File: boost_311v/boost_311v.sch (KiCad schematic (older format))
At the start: 58 parts, among them J2 VO, J3 Vin_boost, Q1 BC556, Q2 PN2222A, Q3 PN2222A, Q4 PN2222A, Q5 IRFP260, Q6 2N3904, Q7 2N3906, U2 L7812, U3 4N25, U4 LF357, U5 NE555

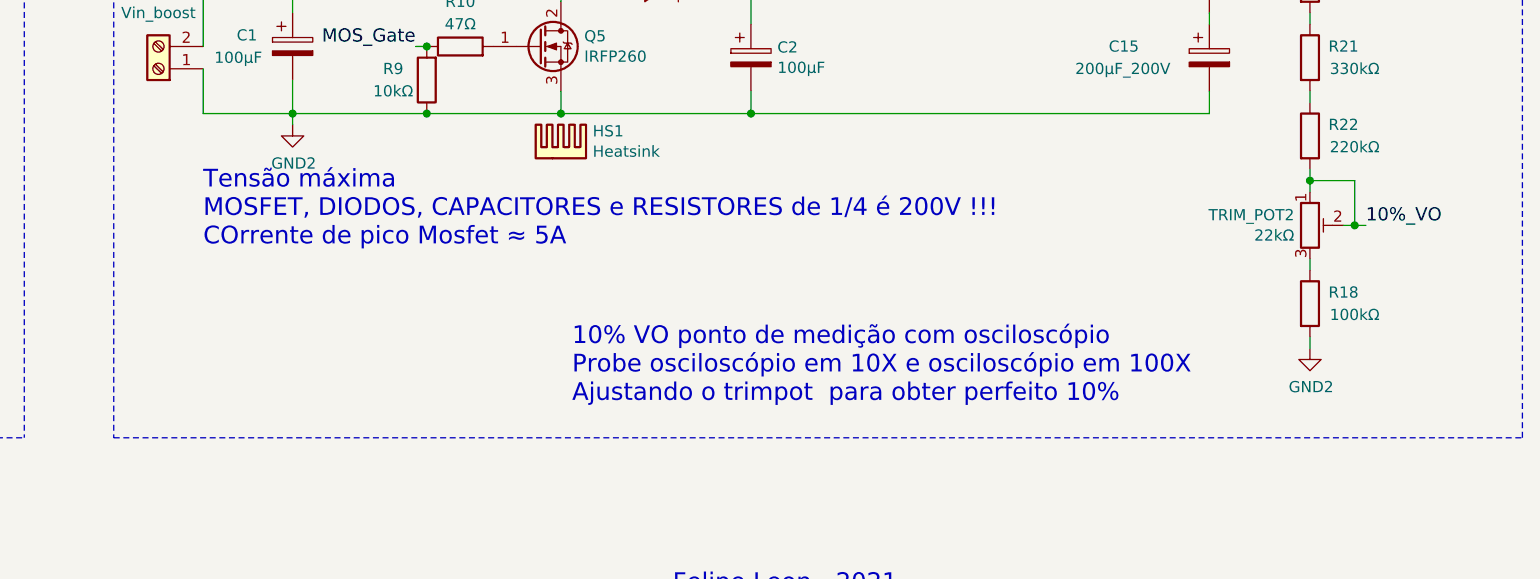
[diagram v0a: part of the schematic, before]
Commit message: Up pcb
Signed-off-by: fgl27 <fglfgl27@gmail.com>
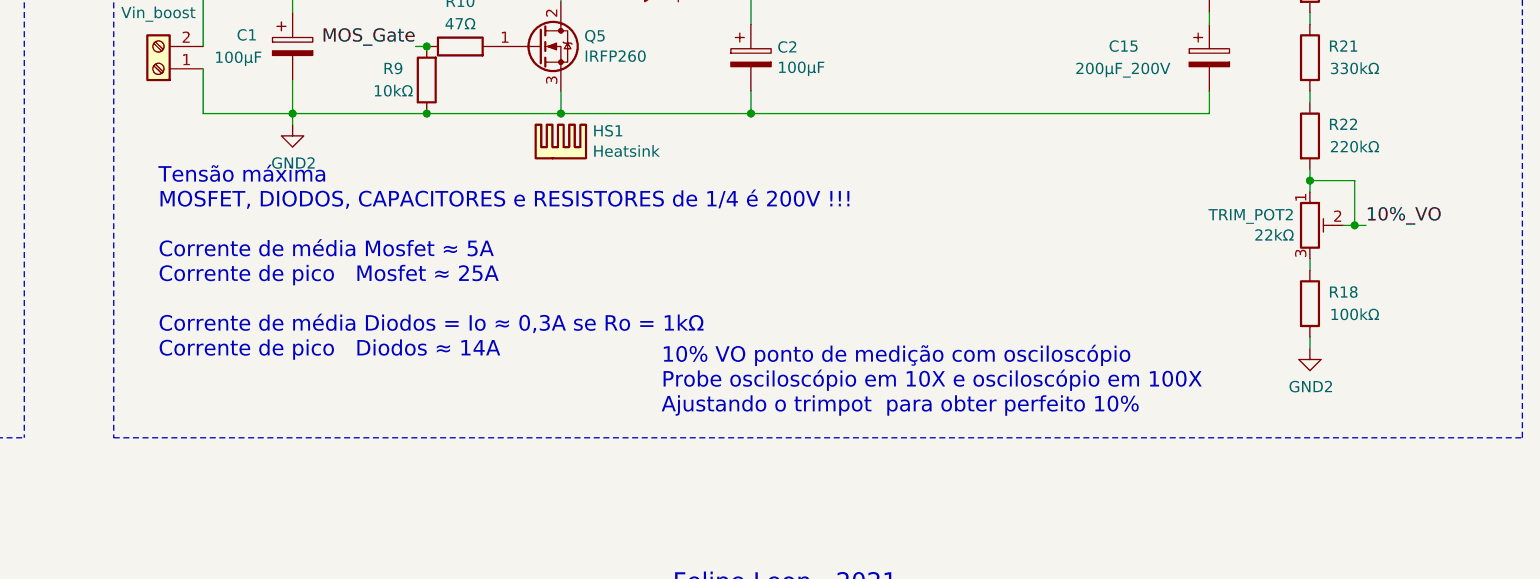
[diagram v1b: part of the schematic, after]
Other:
- note added: "Tensão máxima\nMOSFET, DIODOS, CAPACITORES e RESISTORES de 1/4 é 200V !!!\n\nCorrente de média Mosfet ≈ 5A\nCorrente de pico Mosfet ≈ 25A\n\nCorrente de média Diodos = Io ≈ 0,3A se Ro = 1kΩ\nCorrente de pico Diodos ≈ 14A"
- note removed: "Tensão máxima\nMOSFET, DIODOS, CAPACITORES e RESISTORES de 1/4 é 200V !!!\nCOrrente de pico Mosfet ≈ 5A"
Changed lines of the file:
@@
 	0    -1   -1   0
 $EndComp
-Text Notes 9100 6950 0    79   ~ 0
-                   Tensão máxima\nMOSFET, DIODOS, CAPACITORES e RESISTORES de 1/4 é 200V !!!\nCOrrente de pico Mosfet ≈ 5A
+Text Notes 8900 7450 0    69   ~ 0
+                   Tensão máxima\nMOSFET, DIODOS, CAPACITORES e RESISTORES de 1/4 é 200V !!!\n\nCorrente de média Mosfet ≈ 5A\nCorrente de pico   Mosfet ≈ 25A\n\nCorrente de média Diodos = Io ≈ 0,3A se Ro = 1kΩ\nCorrente de pico   Diodos ≈ 14A
 Text Notes 13950 5150 0    49   ~ 0
 Carga Máxima 0,3A\n1kΩ quando VO = 311V
@@
 Wire Notes Line
 	8700 4350 8700 7800
-Text Notes 10750 7650 0    79   ~ 0
+Text Notes 11150 7700 0    69   ~ 0
 10% VO ponto de medição com osciloscópio\nProbe osciloscópio em 10X e osciloscópio em 100X\nAjustando o trimpot  para obter perfeito 10%
 $Comp

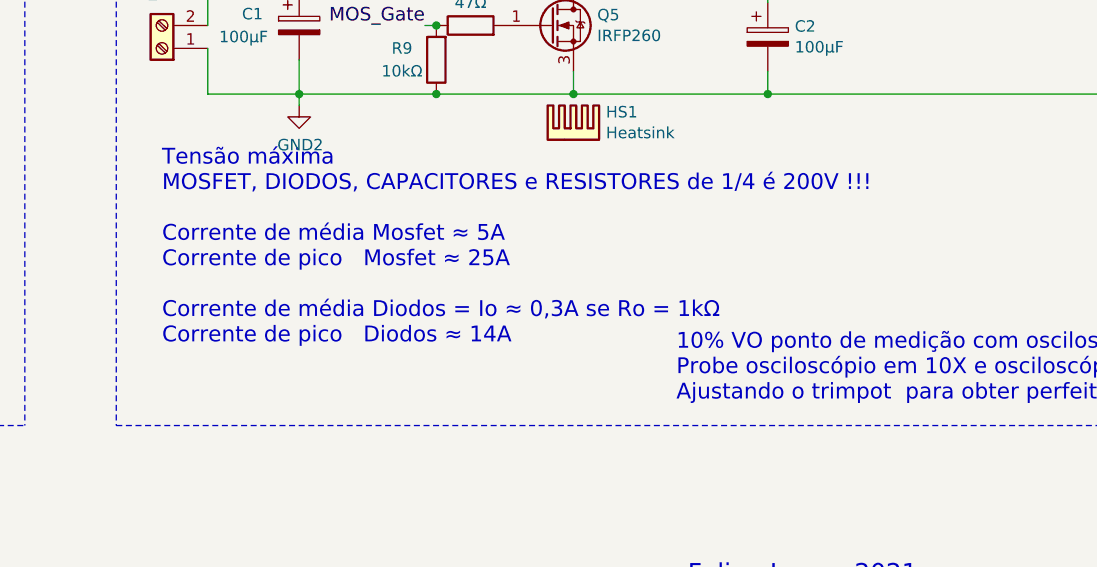
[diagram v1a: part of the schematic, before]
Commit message: Up pcb
Signed-off-by: fgl27 <fglfgl27@gmail.com>
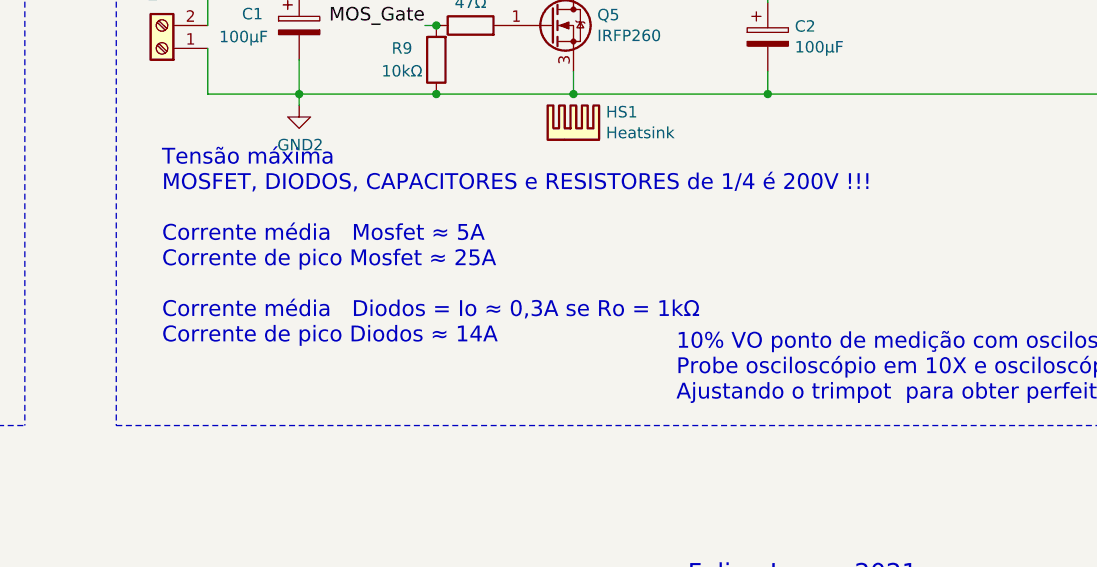
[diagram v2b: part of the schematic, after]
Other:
- note added: "Tensão máxima\nMOSFET, DIODOS, CAPACITORES e RESISTORES de 1/4 é 200V !!!\n\nCorrente média Mosfet ≈ 5A\nCorrente de pico Mosfet ≈ 25A\n\nCorrente média Diodos = Io ≈ 0,3A se Ro = 1kΩ\nCorrente de pico Diodos ≈ 14A"
- note removed: "Tensão máxima\nMOSFET, DIODOS, CAPACITORES e RESISTORES de 1/4 é 200V !!!\n\nCorrente de média Mosfet ≈ 5A\nCorrente de pico Mosfet ≈ 25A\n\nCorrente de média Diodos = Io ≈ 0,3A se Ro = 1kΩ\nCorrente de pico Diodos ≈ 14A"
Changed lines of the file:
@@
 $EndComp
 Text Notes 8900 7450 0    69   ~ 0
-                   Tensão máxima\nMOSFET, DIODOS, CAPACITORES e RESISTORES de 1/4 é 200V !!!\n\nCorrente de média Mosfet ≈ 5A\nCorrente de pico   Mosfet ≈ 25A\n\nCorrente de média Diodos = Io ≈ 0,3A se Ro = 1kΩ\nCorrente de pico   Diodos ≈ 14A
+                   Tensão máxima\nMOSFET, DIODOS, CAPACITORES e RESISTORES de 1/4 é 200V !!!\n\nCorrente média   Mosfet ≈ 5A\nCorrente de pico Mosfet ≈ 25A\n\nCorrente média   Diodos = Io ≈ 0,3A se Ro = 1kΩ\nCorrente de pico Diodos ≈ 14A
 Text Notes 13950 5150 0    49   ~ 0
 Carga Máxima 0,3A\n1kΩ quando VO = 311V
